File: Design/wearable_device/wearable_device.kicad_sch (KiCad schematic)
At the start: 3 parts, among them IC1 TESEO-LIV3R, U1 ESP32-S3-MINI-1, U2 MAX30102

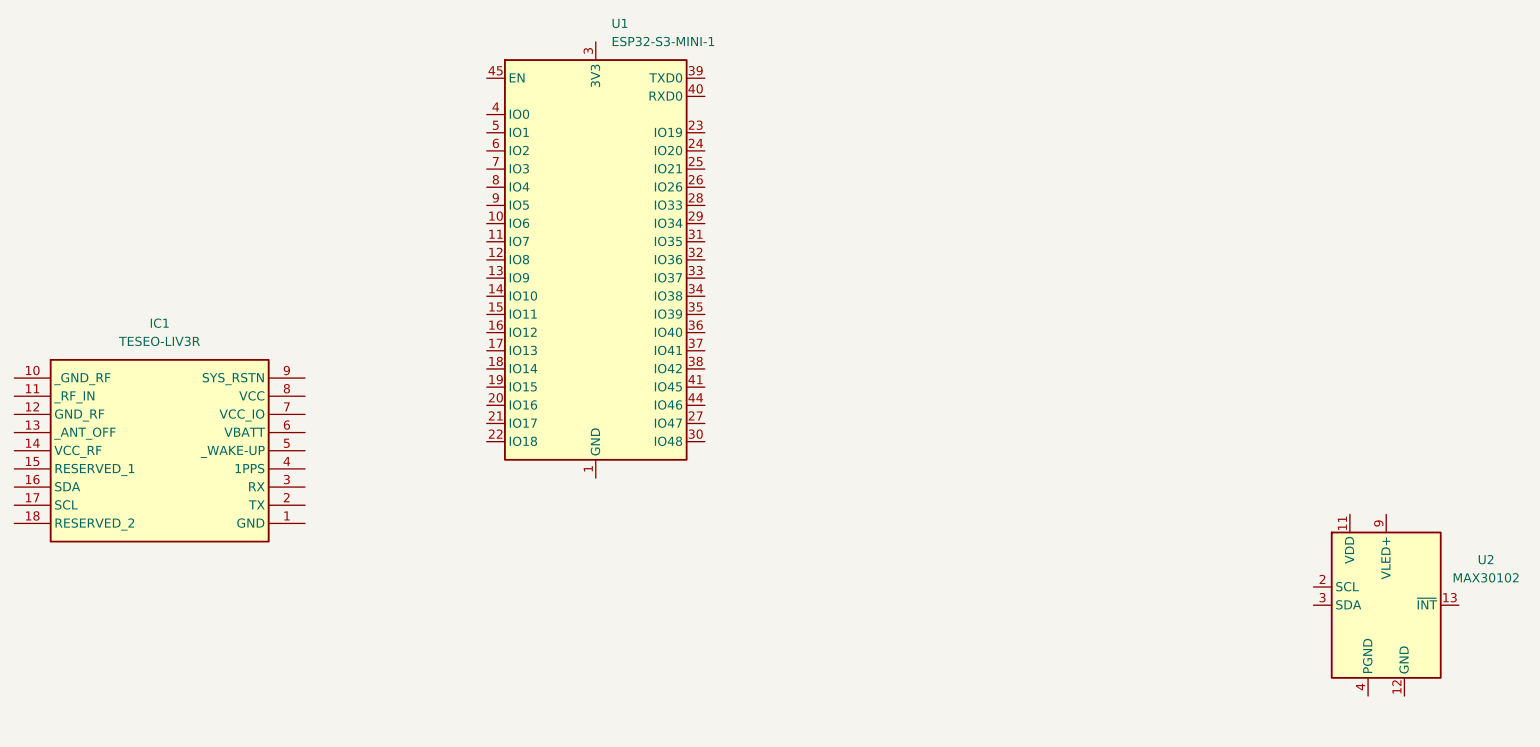
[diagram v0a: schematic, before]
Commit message: add design
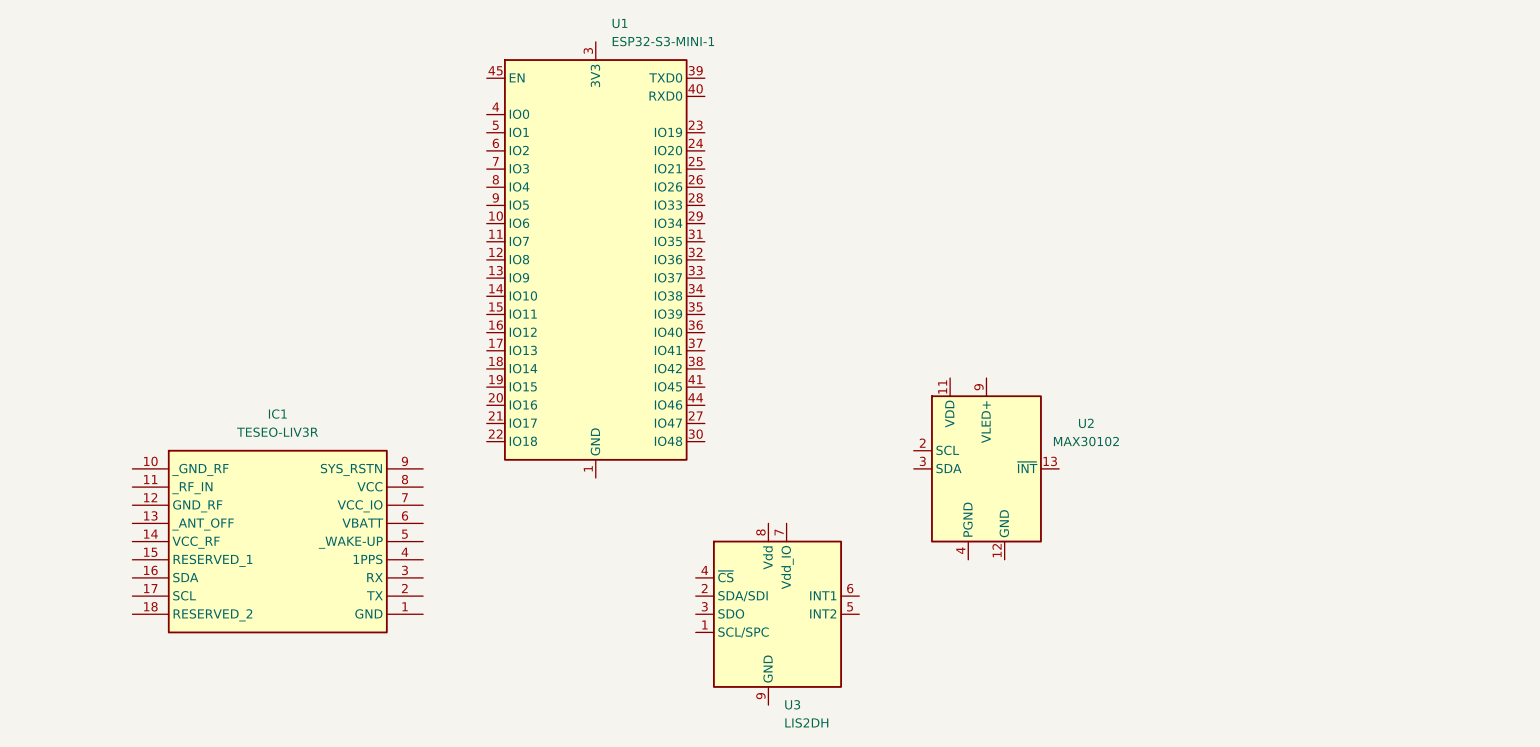
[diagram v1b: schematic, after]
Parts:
- added U3: LIS2DH, Package_LGA:LGA-14_2x2mm_P0.35mm_LayoutBorder3x4y, symbol Sensor_Motion:LIS2DH
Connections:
- new net: U3.10 (GND), U3.11 (GND), U3.12 (GND), U3.13 (GND), U3.14 (GND), U3.9 (GND)
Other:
- moved on the sheet: IC1, U2
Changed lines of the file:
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@@
 	(symbol
 		(lib_id "Sensor:MAX30102")
-		(at 340.36 156.21 0)
+		(at 284.48 137.16 0)
 		(unit 1)
 		(exclude_from_sim no)
@@
 		(fields_autoplaced yes)
 		(property "Reference" "U2"
-			(at 354.33 149.8914 0)
+			(at 298.45 130.8414 0)
 			(effects
 				(font
@@
 		)
 		(property "Value" "MAX30102"
-			(at 354.33 152.4314 0)
+			(at 298.45 133.3814 0)
 			(effects
 				(font
@@
 		)
 		(property "Footprint" "OptoDevice:Maxim_OLGA-14_3.3x5.6mm_P0.8mm"
-			(at 340.36 158.75 0)
+			(at 284.48 139.7 0)
 			(effects
 				(font
@@
 		)
 		(property "Datasheet" "https://datasheets.maximintegrated.com/en/ds/MAX30102.pdf"
-			(at 340.36 156.21 0)
+			(at 284.48 137.16 0)
 			(effects
 				(font
@@
 		)
 		(property "Description" "Heart Rate Sensor, 14-OLGA"
-			(at 340.36 156.21 0)
+			(at 284.48 137.16 0)
 			(effects
 				(font
@@
 	(symbol
 		(lib_id "SamacSys_Parts:TESEO-LIV3R")
-		(at 148.59 124.46 0)
+		(at 165.1 137.16 0)
 		(unit 1)
 		(exclude_from_sim no)
@@
 		(fields_autoplaced yes)
 		(property "Reference" "IC1"
-			(at 168.91 116.84 0)
+			(at 185.42 129.54 0)
 			(effects
 				(font
@@
 		)
 		(property "Value" "TESEO-LIV3R"
-			(at 168.91 119.38 0)
+			(at 185.42 132.08 0)
 			(effects
 				(font
@@
 		)
 		(property "Footprint" "TESEOLIV3R"
-			(at 185.42 219.38 0)
+			(at 201.93 232.08 0)
 			(effects
 				(font
@@
 		)
 		(property "Datasheet" "https://www.st.com/resource/en/datasheet/teseo-liv3r.pdf"
-			(at 185.42 319.38 0)
+			(at 201.93 332.08 0)
 			(effects
 				(font
@@
 		)
 		(property "Description" "- RF Receiver BeiDou, GLONASS, GNSS, GPS 1.561GHz, 1.575MHz -163dBm Not Included 18-LCC (9.7x10.1)"
-			(at 148.59 124.46 0)
+			(at 165.1 137.16 0)
 			(effects
 				(font
@@
 		)
 		(property "Height" "2.3"
-			(at 185.42 519.38 0)
+			(at 201.93 532.08 0)
 			(effects
 				(font
@@
 		)
 		(property "Manufacturer_Name" "STMicroelectronics"
-			(at 185.42 619.38 0)
+			(at 201.93 632.08 0)
 			(effects
 				(font
@@
 		)
 		(property "Manufacturer_Part_Number" "TESEO-LIV3R"
-			(at 185.42 719.38 0)
+			(at 201.93 732.08 0)
 			(effects
 				(font
@@
 		)
 		(property "Mouser Part Number" "511-TESEO-LIV3R"
-			(at 185.42 819.38 0)
+			(at 201.93 832.08 0)
 			(effects
 				(font
@@
 		)
 		(property "Mouser Price/Stock" "https://www.mouser.co.uk/ProductDetail/STMicroelectronics/TESEO-LIV3R?qs=ZSypp649SOXG7EmhCFcBlw%3D%3D"
-			(at 185.42 919.38 0)
+			(at 201.93 932.08 0)
 			(effects
 				(font
@@
 		)
 		(property "Arrow Part Number" "TESEO-LIV3R"
-			(at 185.42 1019.38 0)
+			(at 201.93 1032.08 0)
 			(effects
 				(font
@@
 		)
 		(property "Arrow Price/Stock" "https://www.arrow.com/en/products/teseo-liv3r/stmicroelectronics?region=nac"
-			(at 185.42 1119.38 0)
+			(at 201.93 1132.08 0)
 			(effects
 				(font
@@
 					(unit 1)
 				)
+			)
+		)
+	)
+	(symbol
+		(lib_id "Sensor_Motion:LIS2DH")
+		(at 254 157.48 0)
+		(unit 1)
+		(exclude_from_sim no)
+		(in_bom yes)
+		(on_board yes)
+		(dnp no)
+		(fields_autoplaced yes)
+		(property "Reference" "U3"
+			(at 256.1941 170.18 0)
+			(effects
+				(font
+					(size 1.27 1.27)
+				)
+				(justify left)
+			)
+		)
+		(property "Value" "LIS2DH"
+			(at 256.1941 172.72 0)
+			(effects
+				(font
+					(size 1.27 1.27)
+				)
+				(justify left)
+			)
+		)
+		(property "Footprint" "Package_LGA:LGA-14_2x2mm_P0.35mm_LayoutBorder3x4y"
+			(at 254 168.91 0)
+			(effects
+				(font
+					(size 1.27 1.27)
+				)
+				(hide yes)
+			)
+		)
+		(property "Datasheet" "http://www.st.com/web/en/resource/technical/document/datasheet/DM00042751.pdf"
+			(at 254 172.72 0)
+			(effects
+				(font
+					(size 1.27 1.27)
+				)
+				(hide yes)
+			)
+		)
+		(property "Description" "3-Axis Accelerometer, 2/4/8/16g range, I2C/SPI interface, LGA-14"
+			(at 254 157.48 0)
+			(effects
+				(font
+					(size 1.27 1.27)
+				)
+				(hide yes)
+			)
+		)
+		(pin "4"
+		)
+		(pin "2"
+		)
+		(pin "8"
+		)
+		(pin "5"
+		)
+		(pin "12"
+		)
+		(pin "3"
+		)
+		(pin "10"
+		)
+		(pin "1"
+		)
+		(pin "13"
+		)
+		(pin "14"
+		)
+		(pin "6"
+		)
+		(pin "7"
+		)
+		(pin "9"
+		)
+		(pin "11"
+		)
+		(instances
+			(project "wearable_device"
+				(path "/094ce06f-6434-4293-ac16-ae8f723afcd4"
+					(reference "U3")
+					(unit 1)
+				)
